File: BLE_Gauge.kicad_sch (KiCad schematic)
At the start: 37 parts, among them J1 TagConnect_TC2030-NL, J2 USB_C_Receptacle_PowerOnly_6P, J3 Conn_01x12_MountingPin, Q1 SS8050, U1 nRF54L15-QFXX, U2 LSM6DS3, X1 32MHz, X2 32.768kHz

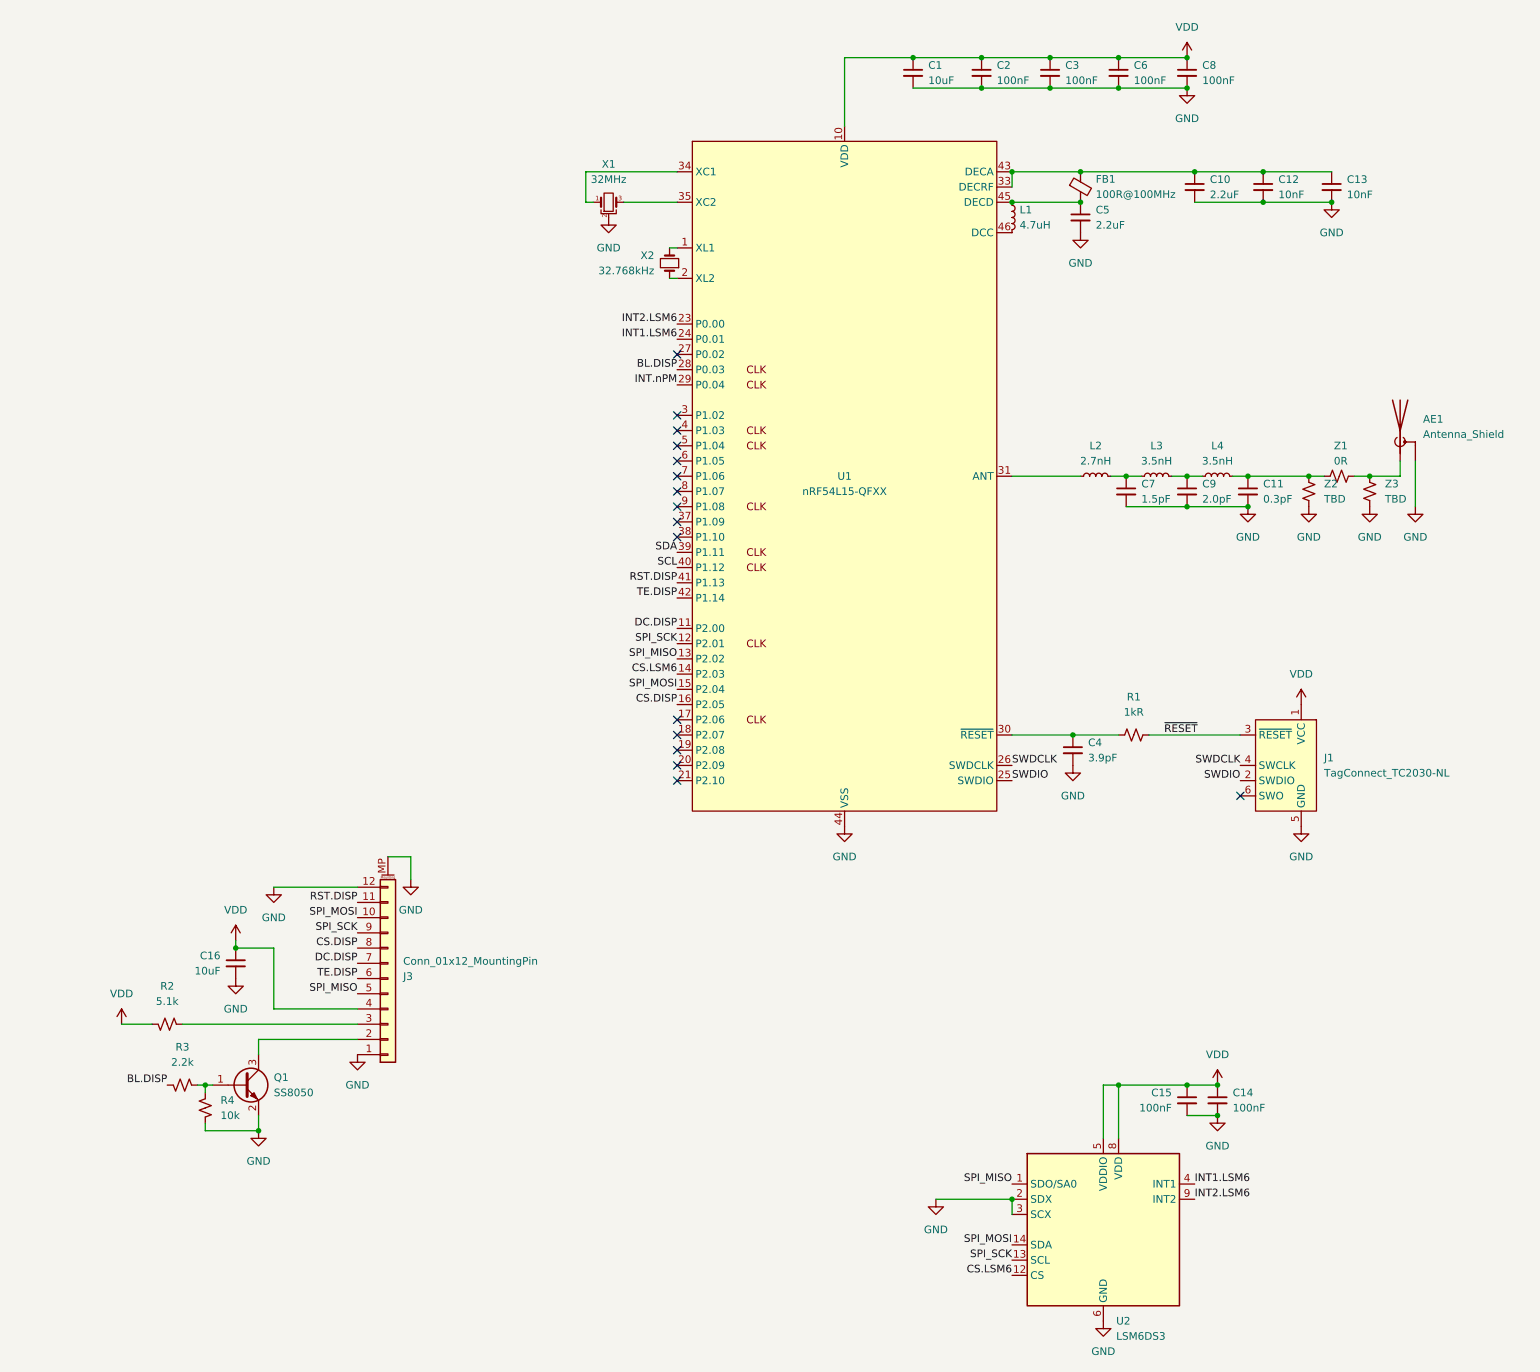
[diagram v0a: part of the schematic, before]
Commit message: Arrumando bagunça
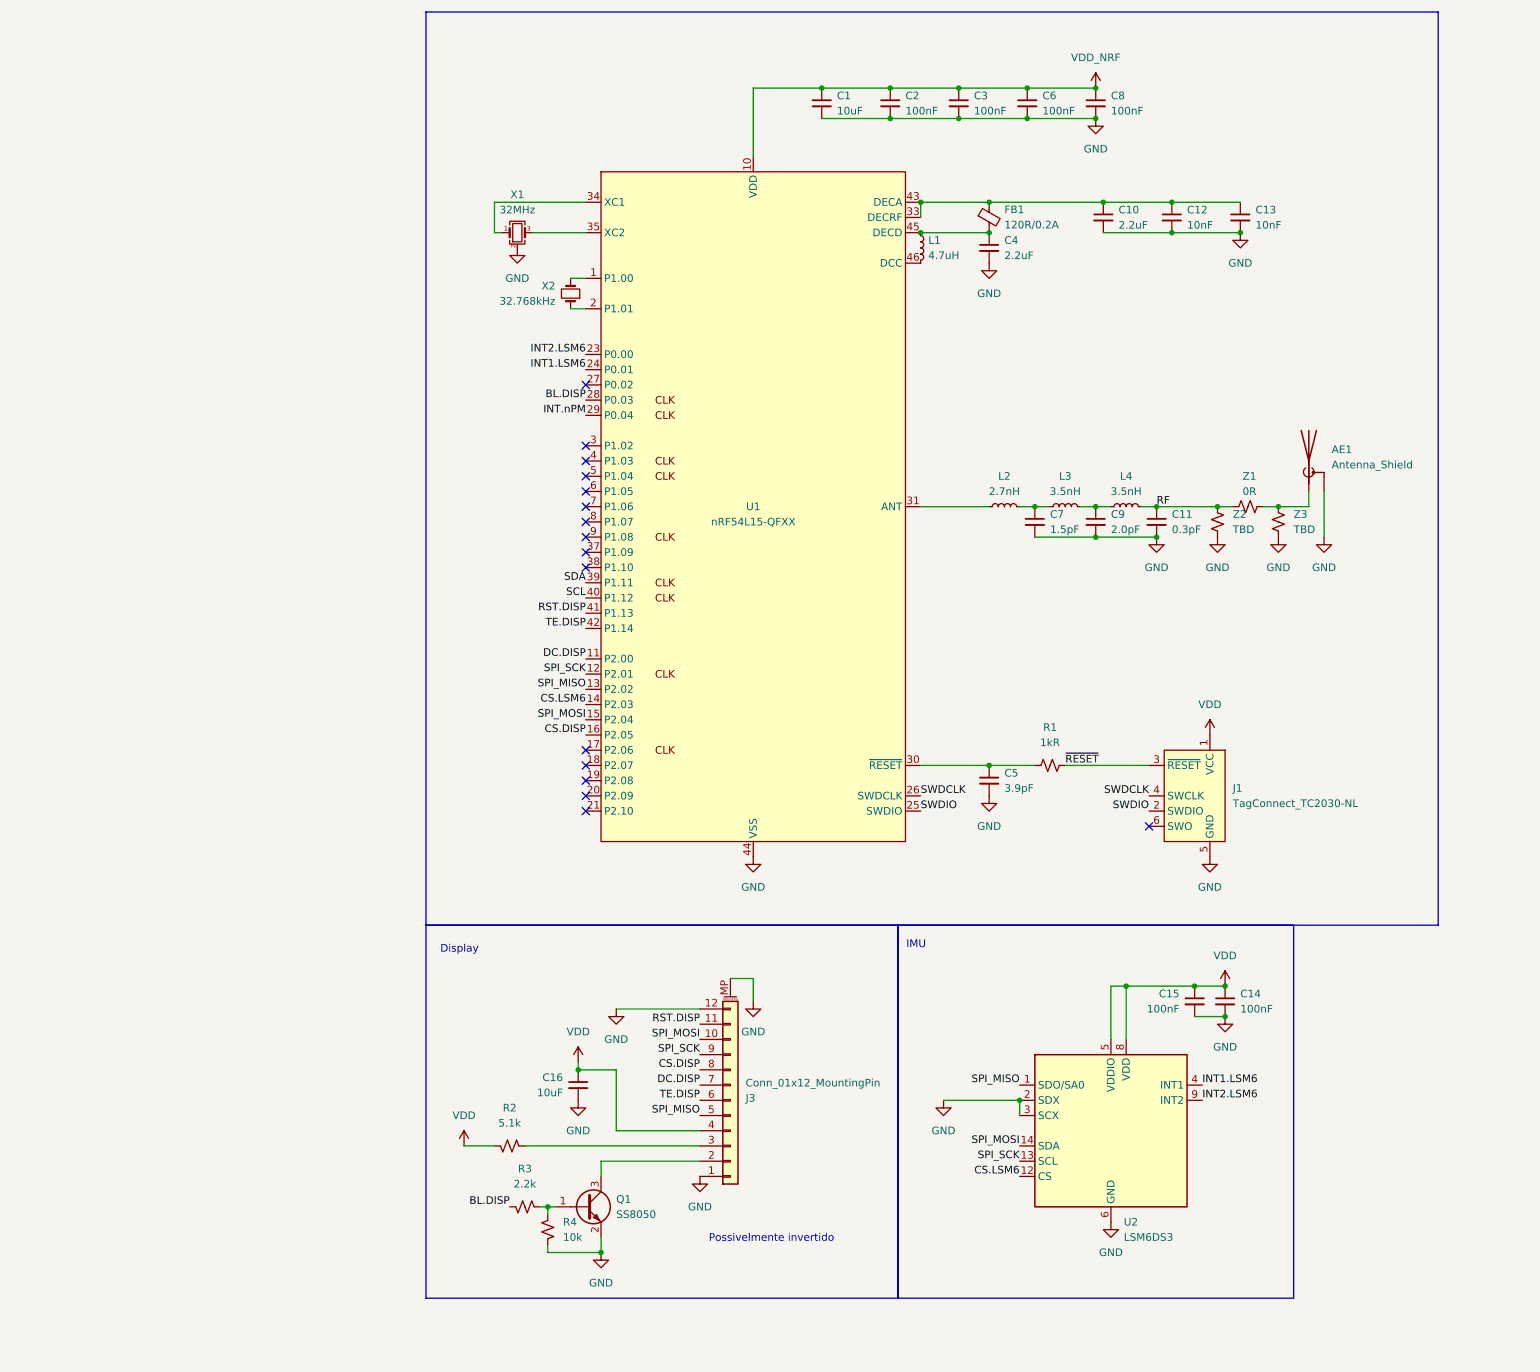
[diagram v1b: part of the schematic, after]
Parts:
- removed X1: 32MHz, Crystal:Crystal_SMD_2016-4Pin_2.0x1.6mm, symbol Device:Crystal_GND2_Small
- added X1: 32MHz, Crystal:Crystal_SMD_2016-4Pin_2.0x1.6mm, symbol Device:Crystal_GND24_Small
- C1: footprint Capacitor_SMD:C_0402_1005Metric -> Nath:C_0402_1005Metric_Nordic
- C10, C11, C12, C13, C2, C3, C6, C7, C8, C9: footprint Capacitor_SMD:C_0201_0603Metric -> Nath:C_0201_0603Metric_Nordic
- C4: renamed from C5; footprint Capacitor_SMD:C_0201_0603Metric -> Nath:C_0201_0603Metric_Nordic
- C5: renamed from C4; footprint Capacitor_SMD:C_0201_0603Metric -> Nath:C_0201_0603Metric_Nordic
- FB1: value 100R@100MHz -> 120R/0.2A; footprint Inductor_SMD:L_0201_0603Metric -> Nath:L_0201_0603Metric_Nordic
- L1: footprint Inductor_SMD:L_0603_1608Metric -> Nath:L_0603_1608Metric_Nordic
- L2, L3, L4: footprint Inductor_SMD:L_0201_0603Metric -> Nath:L_0201_0603Metric_Nordic
- R1: footprint Resistor_SMD:R_0201_0603Metric -> Nath:R_0201_0603Metric_Nordic
- U1: KiLib_Generator (none) -> package/no_lead
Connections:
- net GND: now also X1.2 (G), X1.4 (G)
- net VDD: no longer C1.1, C2.1, C3.1, C6.1, C8.1, U1.10 (VDD), U1.22 (VDD), U1.36 (VDD), U1.47 (VDD), U1.48 (VDD)
- net RF: now reaches C11.1, L4.2, Z1.2, Z2.2
- net at U1.34 (XC1): now also X1.1
- net at U1.35 (XC2): now also X1.3
- new net VDD_NRF: C1.1, C2.1, C3.1, C6.1, C8.1, U1.10 (VDD), U1.22 (VDD), U1.36 (VDD), U1.47 (VDD), U1.48 (VDD)
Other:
- note added: "Display"
- note added: "IMU"
- note added: "Possivelmente invertido"
- moved on the sheet: AE1, C1, C10, C11, C12, C13, C14, C15, C16, C2, C3, C4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
